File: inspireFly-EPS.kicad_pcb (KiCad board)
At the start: 4 copper layers, 88 x 94.5 mm, 126 parts, among them J1 USB4085-GF-A_REVB, J2 Conn_01x02_Pin, J3 FTSH-107-01-L-DV-K-A, Q1 SQJ123ELP-T1_GE3, Q10 SQJA62EP-T1_GE3, Q3 SQJA62EP-T1_GE3, Q4 SQJA62EP-T1_GE3, Q5 SQJA62EP-T1_GE3, Q6 SQJA62EP-T1_GE3, Q7 SQJA62EP-T1_GE3, Q8 SQJA62EP-T1_GE3, Q9 SQJA62EP-T1_GE3, SW1 SW_Push, SW2 SW_Push, SW3 SW_Push, U1 STM32U575RIT6, U2 BQ25750RRVR, U3 TCAN332DCNR, U4 MAX77504AAFC+T, U6 INA180A3IDBVT, U8 TPS63070RNMR, U9 TPS63070RNMR, Y1 Crystal_GND2

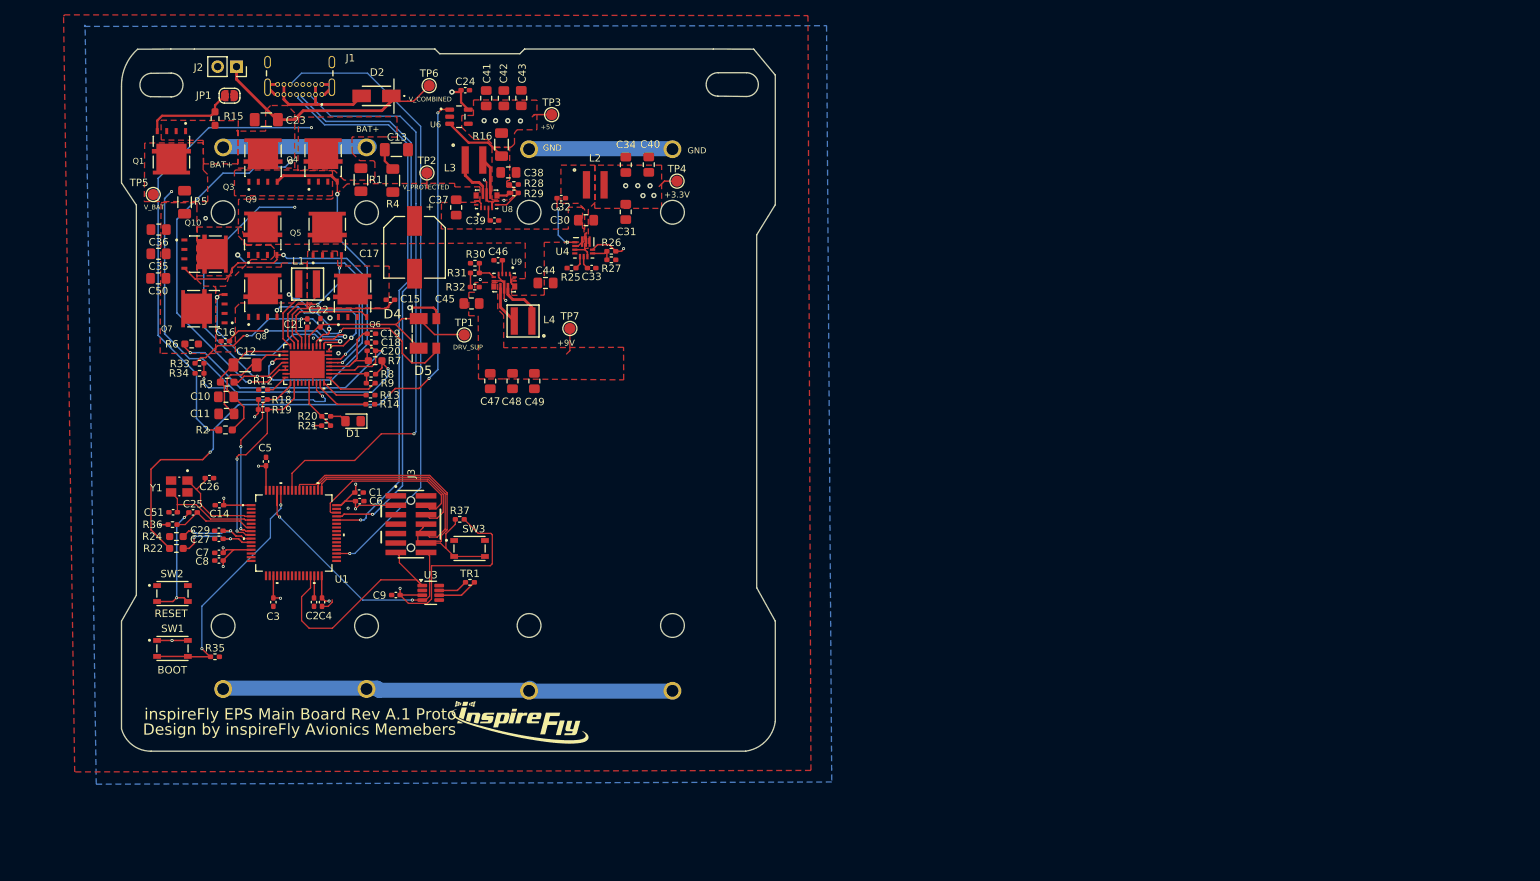
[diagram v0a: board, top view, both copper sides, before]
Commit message: Schematic rework
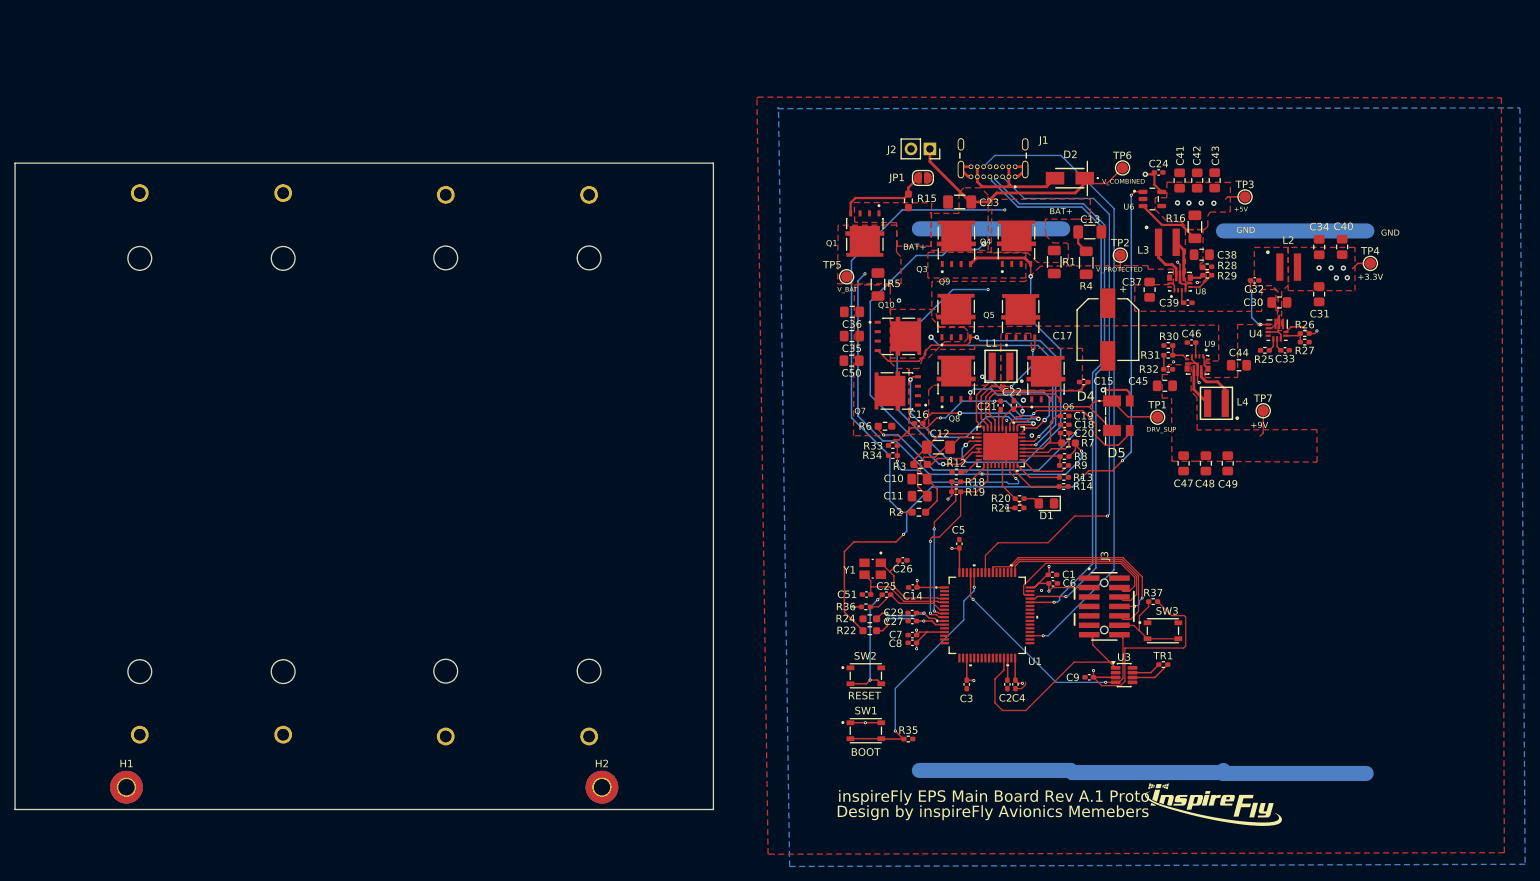
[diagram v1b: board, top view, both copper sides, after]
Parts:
- added H1: MountingHole_Pad, MountingHole:MountingHole_2.2mm_M2_Pad_TopBottom, F.Cu at (38.7, 124.4)
- added H2: MountingHole_Pad, MountingHole:MountingHole_2.2mm_M2_Pad_TopBottom, F.Cu at (102.7, 124.4)
- moved C21 94.0 mm to (156.3, 73.0)
- moved C35 94.0 mm to (136.3, 63.6)
- moved J2 94.0 mm to (146.8, 38.4)
- moved R3 94.0 mm to (145.6, 80.9)
- moved C11 94.0 mm to (145.4, 85.2)
- moved C24 94.0 mm to (177.6, 41.6)
- moved C26 94.0 mm to (143.2, 93.8)
- moved C27 94.0 mm to (144.4, 102.0)
- moved C30 94.0 mm to (193.9, 59.1)
- moved C37 94.0 mm to (176.4, 57.4)
- moved C38 94.0 mm to (183.4, 52.7)
- moved C39 94.0 mm to (181.5, 59.2)
- moved C4 94.0 mm to (158.3, 110.5)
- moved C42 94.0 mm to (182.8, 42.7)
- moved C45 94.0 mm to (178.4, 70.3)
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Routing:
- net SWO: track 34.9 -> 29.1 mm, vias 0 -> 2
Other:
- board size 88 x 94.5 mm -> 94 x 87 mm

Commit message: Routing Updates
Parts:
- removed C1, C18, C19: 100nF, Capacitor_SMD:C_0402_1005Metric_Pad0.74x0.62mm_HandSolder
- removed C10, C11: 100nF, Capacitor_SMD:C_0805_2012Metric_Pad1.18x1.45mm_HandSolder
- removed C12: 470nF, Capacitor_SMD:C_1206_3216Metric_Pad1.33x1.80mm_HandSolder
- removed C13, C23: 2.2uF, Capacitor_SMD:C_1206_3216Metric_Pad1.33x1.80mm_HandSolder
- removed C15, C16: 47nF, Capacitor_SMD:C_0402_1005Metric_Pad0.74x0.62mm_HandSolder
- removed C17: 47uF, inspireFly-EPS-footprints:CAP_EEEFN1J470L
- removed C20: 470nF, Capacitor_SMD:C_0402_1005Metric_Pad0.74x0.62mm_HandSolder
- removed C21, C22: 4.7uF, Capacitor_SMD:C_0402_1005Metric_Pad0.74x0.62mm_HandSolder
- removed C35, C36, C50: 22uF, Capacitor_SMD:C_0805_2012Metric_Pad1.18x1.45mm_HandSolder
- removed C51: 10pF, Capacitor_SMD:C_0402_1005Metric_Pad0.74x0.62mm_HandSolder
- removed D1: LED, Diode_SMD:D_0805_2012Metric_Pad1.15x1.40mm_HandSolder
- removed D4, D5: DFLS130L-7, inspireFly-EPS-footprints:DFLS130L7
- removed G***: LOGO, inspireFly-EPS-footprints:inspireFly_Logo_long
- removed J1: USB4085-GF-A_REVB, inspireFly-EPS-footprints:GCT_USB4085-GF-A_REVB
- removed JP1: BAT_ENABLE, Jumper:SolderJumper-2_P1.3mm_Open_RoundedPad1.0x1.5mm
- removed L1: 2.2uH, inspireFly-EPS-footprints:WE-MXGI_4020
- removed Q1: SQJ123ELP-T1_GE3, inspireFly-EPS-footprints:TRANS_SQJA62EP-T1_GE3
- removed Q10, Q3, Q4, Q5, Q6, Q7, Q8, Q9: SQJA62EP-T1_GE3, inspireFly-EPS-footprints:TRANS_SQJA62EP-T1_GE3
- removed R1, R5: 5m, Resistor_SMD:R_1206_3216Metric_Pad1.30x1.75mm_HandSolder
- removed R12: 40k, Resistor_SMD:R_0402_1005Metric_Pad0.72x0.64mm_HandSolder
- removed R13: 3.3k, Resistor_SMD:R_0402_1005Metric_Pad0.72x0.64mm_HandSolder
- removed R14: 12.5k, Resistor_SMD:R_0402_1005Metric_Pad0.72x0.64mm_HandSolder
- removed R15: 47k, Resistor_SMD:R_0603_1608Metric_Pad0.98x0.95mm_HandSolder
- removed R18, R19: 10k, Resistor_SMD:R_0402_1005Metric_Pad0.72x0.64mm_HandSolder
- removed R2, R3, R6, R7: 10, Resistor_SMD:R_0603_1608Metric_Pad0.98x0.95mm_HandSolder
- removed R20: 330, Resistor_SMD:R_0402_1005Metric_Pad0.72x0.64mm_HandSolder
- removed R21, R33, R34, R35, R36: 10K, Resistor_SMD:R_0402_1005Metric_Pad0.72x0.64mm_HandSolder
- removed R4: 2, Resistor_SMD:R_1206_3216Metric_Pad1.30x1.75mm_HandSolder
- removed R8: 200k, Resistor_SMD:R_0402_1005Metric_Pad0.72x0.64mm_HandSolder
- removed R9: 44.8k, Resistor_SMD:R_0402_1005Metric_Pad0.72x0.64mm_HandSolder
- removed SW1, SW2: SW_Push, inspireFly-EPS-footprints:SW_PTS810_SJM_250_SMTR_LFS
- removed TP1: DRV_SUP, TestPoint:TestPoint_Pad_D1.5mm
- removed TP2: V_PROTECTED, TestPoint:TestPoint_Pad_D1.5mm
- removed TP5: V_BAT, TestPoint:TestPoint_Pad_D1.5mm
- removed U1: STM32U575RIT6, inspireFly-EPS-footprints:LQFP64-10x10mm_STM
- removed U2: BQ25750RRVR, inspireFly-EPS-footprints:VQFN36_RRV_TEX
- removed Y1: Crystal_GND2, inspireFly-EPS-footprints:XTAL_TSX-3225_16.0000MF18X-AC0
- added C53: 100nF, Capacitor_SMD:C_0402_1005Metric_Pad0.74x0.62mm_HandSolder, F.Cu at (70.3, 60.6)
- added C54: 470nF, Capacitor_SMD:C_0402_1005Metric_Pad0.74x0.62mm_HandSolder, F.Cu at (71.7, 59.3)
- added C55: 100nF, Capacitor_SMD:C_0402_1005Metric_Pad0.74x0.62mm_HandSolder, F.Cu at (69.8, 58.6)
- added C57: 4.7uF, Capacitor_SMD:C_0402_1005Metric_Pad0.74x0.62mm_HandSolder, F.Cu at (77.6, 55.4)
- added C58: 4.7uF, Capacitor_SMD:C_0402_1005Metric_Pad0.74x0.62mm_HandSolder, F.Cu at (74.9, 55.3)
- added C59: 1uF, Capacitor_SMD:C_0402_1005Metric_Pad0.74x0.62mm_HandSolder, F.Cu at (69.3, 63.9)
- added C61: 100nF, Capacitor_SMD:C_0402_1005Metric_Pad0.74x0.62mm_HandSolder, F.Cu at (73.4, 55.4)
- added C62: 100nF, Capacitor_SMD:C_0402_1005Metric_Pad0.74x0.62mm_HandSolder, F.Cu at (79.9, 55.3)
- added C63: 100nF, Capacitor_SMD:C_0402_1005Metric_Pad0.74x0.62mm_HandSolder, F.Cu at (84.1, 58.5)
- added C64: 470nF, Capacitor_SMD:C_0402_1005Metric_Pad0.74x0.62mm_HandSolder, F.Cu at (81.0, 60.0)
- added C65: 100nF, Capacitor_SMD:C_0402_1005Metric_Pad0.74x0.62mm_HandSolder, F.Cu at (84.1, 59.6)
- added C66: 10nF, Capacitor_SMD:C_0402_1005Metric_Pad0.74x0.62mm_HandSolder, F.Cu at (40.1, 48.9)
- added C68: 10nF, Capacitor_SMD:C_0402_1005Metric_Pad0.74x0.62mm_HandSolder, F.Cu at (35.7, 48.9)
- added C69: 22uF, Capacitor_SMD:C_0805_2012Metric_Pad1.18x1.45mm_HandSolder, F.Cu at (30.9, 50.4)
- added C70: 22uF, Capacitor_SMD:C_0805_2012Metric_Pad1.18x1.45mm_HandSolder, F.Cu at (30.9, 48.1)
- added C71: 22uF, Capacitor_SMD:C_0805_2012Metric_Pad1.18x1.45mm_HandSolder, F.Cu at (62.1, 79.5)
- added C72: 22uF, Capacitor_SMD:C_0805_2012Metric_Pad1.18x1.45mm_HandSolder, F.Cu at (62.1, 81.9)
- added C73: 22uF, Capacitor_SMD:C_0805_2012Metric_Pad1.18x1.45mm_HandSolder, F.Cu at (62.1, 74.8)
- added C74: 22uF, Capacitor_SMD:C_0805_2012Metric_Pad1.18x1.45mm_HandSolder, F.Cu at (62.1, 77.0)
- added C75: 22uF, Capacitor_SMD:C_0805_2012Metric_Pad1.18x1.45mm_HandSolder, F.Cu at (47.1, 53.8)
- added C76: 22uF, Capacitor_SMD:C_0805_2012Metric_Pad1.18x1.45mm_HandSolder, F.Cu at (47.1, 50.4)
- added C77: 22uF, Capacitor_SMD:C_0805_2012Metric_Pad1.18x1.45mm_HandSolder, F.Cu at (48.3, 46.2)
- added C78: 22uF, Capacitor_SMD:C_0805_2012Metric_Pad1.18x1.45mm_HandSolder, F.Cu at (45.1, 46.2)
- added C79: 22uF, Capacitor_SMD:C_0805_2012Metric_Pad1.18x1.45mm_HandSolder, F.Cu at (30.9, 45.9)
- added C80: 22uF, Capacitor_SMD:C_0805_2012Metric_Pad1.18x1.45mm_HandSolder, F.Cu at (58.8, 57.0)
- added D3: LTST-S270KRKT, LED_SMD:LED_0603_1608Metric_Pad1.05x0.95mm_HandSolder, F.Cu at (78.0, 67.3)
- added J5: USB4110-GF-A, inspireFly-EPS-footprints:USB4110-GF-A_GCT, F.Cu at (71.4, 45.0)
- added JP2: FTSW EN, Jumper:SolderJumper-2_P1.3mm_Open_TrianglePad1.0x1.5mm, F.Cu at (28.5, 43.1)
- added L5: 10uH, inspireFly-EPS-footprints:WE-XHMA_1090, F.Cu at (49.5, 64.3)
- added Q14: SQJA62EP-T1_GE3, inspireFly-EPS-footprints:TRANS_SQJA62EP-T1_GE3, F.Cu at (61.1, 70.0)
- added Q15: SQJA62EP-T1_GE3, inspireFly-EPS-footprints:TRANS_SQJA62EP-T1_GE3, F.Cu at (52.7, 74.3)
- added Q16: SQJA62EP-T1_GE3, inspireFly-EPS-footprints:TRANS_SQJA62EP-T1_GE3, F.Cu at (53.2, 54.0)
- added Q17: SQJA62EP-T1_GE3, inspireFly-EPS-footprints:TRANS_SQJA62EP-T1_GE3, F.Cu at (61.1, 62.1)
- added R10: 390k, Resistor_SMD:R_0402_1005Metric, F.Cu at (35.4, 42.4)
- added R11: 110k, Resistor_SMD:R_0402_1005Metric, F.Cu at (33.0, 42.4)
- added R17: 47k, Resistor_SMD:R_0402_1005Metric_Pad0.72x0.64mm_HandSolder, F.Cu at (81.6, 62.9)
- added R38: 210k, Resistor_SMD:R_0402_1005Metric_Pad0.72x0.64mm_HandSolder, F.Cu at (81.6, 61.7)
- added R39: 10, Resistor_SMD:R_0402_1005Metric_Pad0.72x0.64mm_HandSolder, F.Cu at (68.3, 60.8)
- added R40: 6.2k, Resistor_SMD:R_0402_1005Metric_Pad0.72x0.64mm_HandSolder, F.Cu at (81.6, 65.3)
- added R41: 36k, Resistor_SMD:R_0402_1005Metric_Pad0.72x0.64mm_HandSolder, F.Cu at (81.6, 66.4)
- added R42: 5m, Resistor_SMD:R_1206_3216Metric_Pad1.30x1.75mm_HandSolder, F.Cu at (58.3, 77.7)
- added R43: 15k, Resistor_SMD:R_0402_1005Metric_Pad0.72x0.64mm_HandSolder, F.Cu at (81.6, 64.2)
- added R44: 40k, Resistor_SMD:R_0402_1005Metric_Pad0.72x0.64mm_HandSolder, F.Cu at (71.5, 63.2)
- added R45: 10, Resistor_SMD:R_0402_1005Metric_Pad0.72x0.64mm_HandSolder, F.Cu at (66.1, 60.8)
- added R46: 10k, Resistor_SMD:R_0402_1005Metric_Pad0.72x0.64mm_HandSolder, F.Cu at (75.3, 65.2)
- added R47: 10k, Resistor_SMD:R_0402_1005Metric_Pad0.72x0.64mm_HandSolder, F.Cu at (77.6, 65.2)
- added R48: 10, Resistor_SMD:R_0402_1005Metric_Pad0.72x0.64mm_HandSolder, F.Cu at (76.2, 55.4)
- added R49: 10, Resistor_SMD:R_0402_1005Metric_Pad0.72x0.64mm_HandSolder, F.Cu at (84.1, 57.3)
- added R50: 5m, Resistor_SMD:R_1206_3216Metric_Pad1.30x1.75mm_HandSolder, F.Cu at (52.4, 46.4)
- added R51: 10, Resistor_SMD:R_0402_1005Metric_Pad0.72x0.64mm_HandSolder, F.Cu at (84.1, 60.6)
- added R52: 680, Resistor_SMD:R_0402_1005Metric_Pad0.72x0.64mm_HandSolder, F.Cu at (37.9, 48.9)
- added R53: 390k, Resistor_SMD:R_0402_1005Metric, F.Cu at (35.5, 43.7)
- added R54: 100k, Resistor_SMD:R_0402_1005Metric_Pad0.72x0.64mm_HandSolder, F.Cu at (138.1, 69.8)
- added RN1: YC158TJR-072K2L, inspireFly-EPS-footprints:RESCAXE64P320X160X70-10N, F.Cu at (141.3, 50.4)
- added SW4: SW_TL1015AF160QG, inspireFly-EPS-footprints:SW_TL1015AF160QG, F.Cu at (134.3, 79.0)
- added U10: BQ25756ERRVR, inspireFly-EPS-footprints:IC_BQ25756ERRVR, F.Cu at (76.5, 60.6)
- added U13: TPS259472ARPWR, inspireFly-EPS-footprints:RPW0010A-MFG, F.Cu at (36.7, 46.0)
- added U5: STM32U575CIT6, inspireFly-EPS-footprints:LQFP48-7x7mm_STM, F.Cu at (156.2, 52.5)
- added Y2: XTAL_ABS07-32.768KHZ-T, inspireFly-EPS-footprints:XTAL_ABS07-32.768KHZ-T, F.Cu at (171.9, 54.3)
- C25: value 100nF -> 22pF
- C26: value 10pF -> 22pF
- C6: value 10uF -> 1uF
- R37: value 10K -> 10k
- SW3: value SW_Push -> SW_TL1015AF160QG; footprint inspireFly-EPS-footprints:SW_PTS810_SJM_250_SMTR_LFS -> inspireFly-EPS-footprints:SW_TL1015AF160QG
- moved C40 229.8 mm to (-20.9, 106.4), turned to 0 degrees
- moved C34 224.8 mm to (-20.9, 97.3), turned to 0 degrees
- moved C31 223.1 mm to (-20.9, 94.3), turned to 0 degrees
- moved TP4 222.6 mm to (-14.3, 84.9)
- moved C44 218.4 mm to (-22.5, 124.5)
- moved C46 217.5 mm to (-21.6, 141.0), turned to 0 degrees
- moved C30 217.2 mm to (-20.9, 91.3)
- moved C49 216.7 mm to (-22.5, 136.5), turned to 0 degrees
- moved TP7 213.8 mm to (-15.9, 125.0)
- moved C48 213.1 mm to (-22.5, 133.5), turned to 0 degrees
- moved R27 212.8 mm to (-12.8, 98.5), turned to 0 degrees
- moved U4 212.8 mm to (-15.5, 102.4)
- moved R26 212.7 mm to (-12.8, 96.5)
- moved C47 209.4 mm to (-22.5, 130.5), turned to 0 degrees
- moved C45 208.9 mm to (-22.5, 127.5), turned to 0 degrees
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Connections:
- net BAT + renamed BAT+
- net V_BUS_COMBINED renamed EXTERNAL_VOLTAGE
- net V_PROTECTED renamed PROTECTED_VOLTAGE
- C25 pad 1: Net-(U1A-NRST) -> GND
- J3 pad 13: CAN_TX -> DEBUG_LPUART_TX
- J3 pad 14: CAN_RX -> DEBUG_LPUART_RX
- R37 pad 1: NRST -> +3.3V
- R37 pad 2: +3.3V -> NRST
- SW3 pad 1: GND -> NRST
- SW3 pad 2: NRST -> GND
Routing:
- net Net-(U6-OUT): track 93.7 -> 0.00 mm, vias 4 -> 0
- net +3.3V: track 88.7 -> 0.00 mm, vias 20 -> 0
- net USB_CC2: track 84.8 -> 0.00 mm, vias 1 -> 0
- net USB_CC1: track 78.1 -> 0.00 mm, vias 1 -> 0
- net USB_D+: track 75.0 -> 0.00 mm, vias 1 -> 0
- net USB_D-: track 74.6 -> 0.00 mm, vias 1 -> 0
- net EXTERNAL_VOLTAGE: track 84.6 -> 20.1 mm, vias 2 -> 13
- net Net-(Q4-D): track 61.6 -> 0.00 mm, vias 2 -> 0
- net Net-(BT1-Pad1-): track 60.4 -> 0.00 mm
- net Net-(Q1-D): track 58.4 -> 0.00 mm, vias 2 -> 0
- net Net-(Q3-G): track 51.7 -> 0.00 mm, vias 2 -> 0
- net EXTERNAL_SIDE_INDUC: track 0.00 -> 50.0 mm, vias 0 -> 2
- net PROTECTED_VOLTAGE: track 48.6 -> 0.00 mm, vias 2 -> 0
- net EXTERNAL_HIGH_SIDE_DRIVE: track 0.00 -> 47.6 mm, vias 0 -> 2
- net GND: track 55.8 -> 13.0 mm
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- added copper zone on F.Cu, net BAT_SIDE_INDUC
- added copper zone on F.Cu, net EXTERNAL_SIDE_INDUC
- added copper zone on In2.Cu, net EXTERNAL_VOLTAGE
- added copper zone on B.Cu, net Net-(BT1-Pad1-)
- added copper zone on F.Cu, net Net-(Q14-D)
- added copper zone on F.Cu, net Net-(Q16-D)
- removed copper zone on F.Cu, net +3.3V
- removed copper zone on In2.Cu, net +3.3V
- removed copper zone on F.Cu, net +5V
- removed copper zone on In2.Cu, net +5V
- removed copper zone on F.Cu, net +9V
- removed copper zone on F.Cu, net Net-(Q1-D)
- removed copper zone on F.Cu, net Net-(Q10-D)
- removed copper zone on F.Cu, net Net-(Q10-S)
- removed copper zone on F.Cu, net Net-(Q3-S)
- removed copper zone on F.Cu, net Net-(Q4-D)
- removed copper zone on F.Cu, net Net-(Q5-S)
- removed copper zone on F.Cu, net Net-(Q7-S)
- removed copper zone on F.Cu, net Net-(U4-LX)
- removed copper zone on F.Cu, net Net-(U6-IN+)
- removed copper zone on F.Cu, net PROTECTED_VOLTAGE
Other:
- board text removed: "+3.3V"
- board text removed: "+5V"
- board text removed: "+9V"
- board text removed: "BAT+"
- board text removed: "BOOT"
- board text removed: "DRV_SUP"
- board text removed: "Design by inspireFly Avionics Memebers"
- board text removed: "GND"
- board text removed: "RESET"
- board text removed: "V_BAT"
- board text removed: "V_COMBINED"
- board text removed: "V_PROTECTED"
- board text removed: "inspireFly EPS Main Board Rev A.1 Proto"
